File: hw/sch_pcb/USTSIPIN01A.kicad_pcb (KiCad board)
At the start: 2 copper layers, 90.9 x 50.3 mm, 112 parts, among them J1 HEADER_2x01_PARALLEL, J19 HEADER_2x01_PARALLEL, J2 HEADER_2x01_PARALLEL, J22 HEADER_2x03, J3 HEADER_2x01_PARALLEL, J4 HEADER_1x01, J5 HEADER_1x01, J6 HEADER_1x01, J7 HEADER_1x01, M1 HOLE, M2 HOLE, M3 HOLE, M4 HOLE, M5 BMI-S-210-F, M6 BMI-S-210-F, M7 BMI-S-210-F, M8 BMI-S-204-F, U1 OPA2314, U10 ATMEGA1284P-AU, U11 PCF85263A, U2 OPA2314, U3 ISL21080DIH312Z-TK 1V25, U4 TS7211, U5 TS5A4594, U6 TPS613221ADBV, U8 TPS613222ADBV, Y1 16MHz, Y2 ABS07-120-32.768KHZ-T

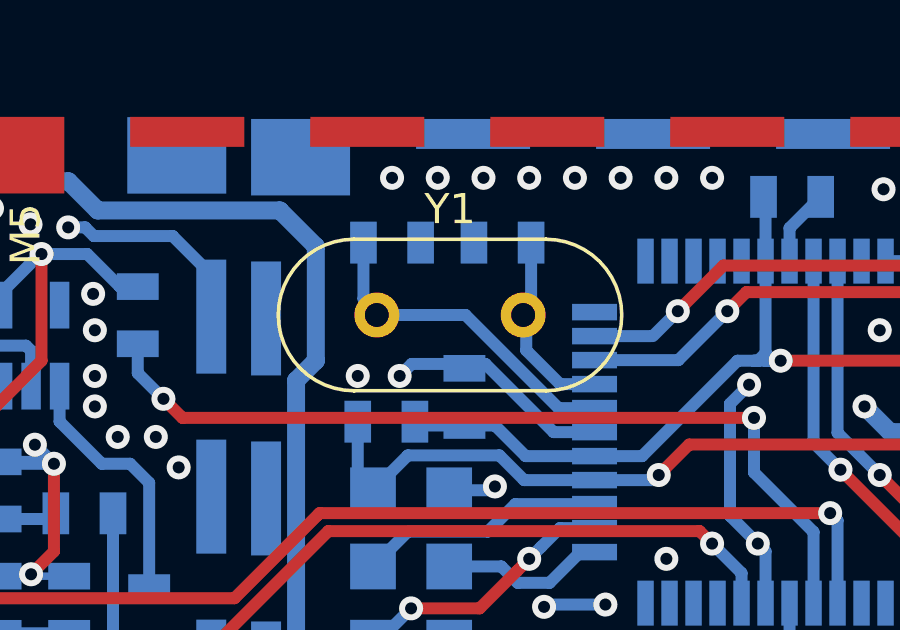
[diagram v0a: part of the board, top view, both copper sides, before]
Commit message: Edit schema
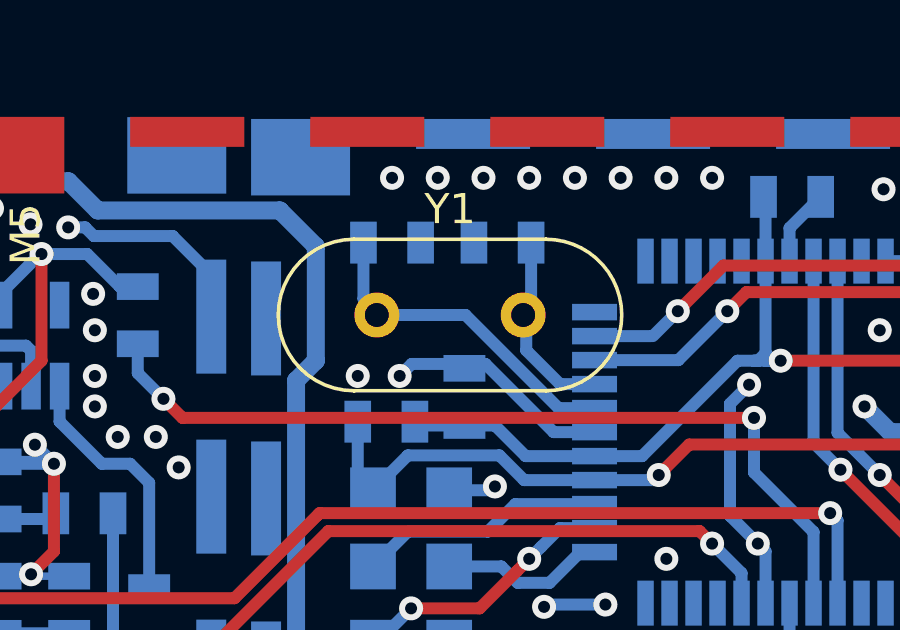
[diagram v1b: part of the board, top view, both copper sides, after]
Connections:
- C24 pad 1: /K -> /Ubiasout
- R22 pad 1: /K -> /Ubiasout
- U10 pad 11: (no net) -> unconnected-(U10-Pad11)
- U10 pad 12: (no net) -> unconnected-(U10-Pad12)
- U10 pad 13: (no net) -> unconnected-(U10-Pad13)
- U10 pad 14: (no net) -> unconnected-(U10-Pad14)
- U10 pad 15: (no net) -> unconnected-(U10-Pad15)
- U10 pad 16: (no net) -> unconnected-(U10-Pad16)
- U10 pad 21: (no net) -> unconnected-(U10-Pad21)
- U10 pad 23: (no net) -> unconnected-(U10-Pad23)
- U10 pad 24: (no net) -> unconnected-(U10-Pad24)
- U10 pad 25: (no net) -> unconnected-(U10-Pad25)
- U10 pad 30: (no net) -> unconnected-(U10-Pad30)
- U10 pad 31: (no net) -> unconnected-(U10-Pad31)
- U10 pad 32: (no net) -> unconnected-(U10-Pad32)
- U10 pad 33: (no net) -> unconnected-(U10-Pad33)
- U10 pad 34: (no net) -> unconnected-(U10-Pad34)
- U10 pad 35: (no net) -> unconnected-(U10-Pad35)
- U10 pad 41: (no net) -> unconnected-(U10-Pad41)
- U10 pad 42: (no net) -> unconnected-(U10-Pad42)
- U10 pad 43: (no net) -> unconnected-(U10-Pad43)
- U10 pad 44: (no net) -> unconnected-(U10-Pad44)
- U11 pad 4: (no net) -> unconnected-(U11-Pad4)
- U11 pad 8: (no net) -> unconnected-(U11-Pad8)
- U11 pad 9: (no net) -> unconnected-(U11-Pad9)
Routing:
- net /Ubiasout: track 0.00 -> 5.94 mm
- net /K: track 5.94 -> 0.00 mm
